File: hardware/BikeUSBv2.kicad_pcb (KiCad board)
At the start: 2 copper layers, 43.6 x 25.5 mm, 53 parts, among them J1 TYPE-C-31-M-16, J2 JST S2B-EH(LF)(SN), SW1 1TS002E-2500-2501-CT, SW2 1TS002E-2500-2501-CT, U1 TPS63020DSJR, U2 ATtiny1616-M, U3 FUSB302B10MPX, U4 HT7550-2, U5 TPS25200

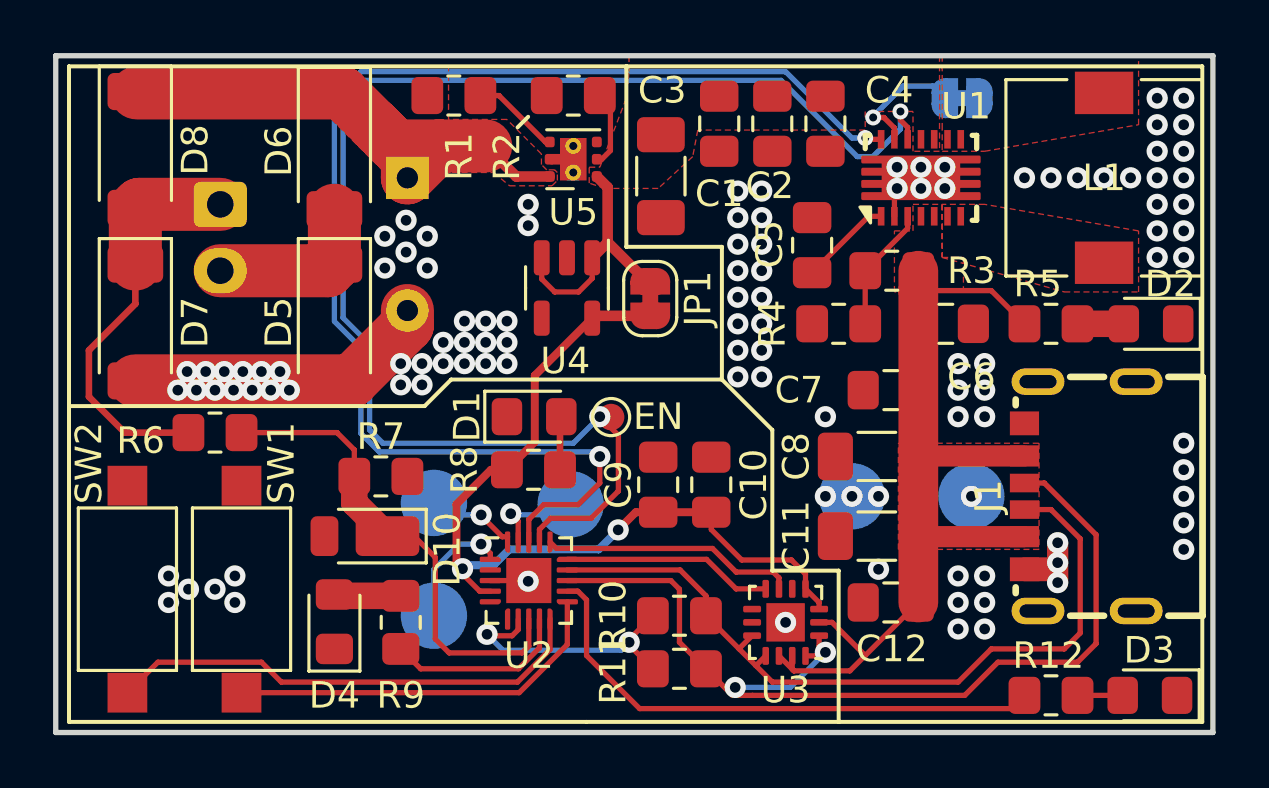
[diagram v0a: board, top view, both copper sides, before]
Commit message: auto cleanup
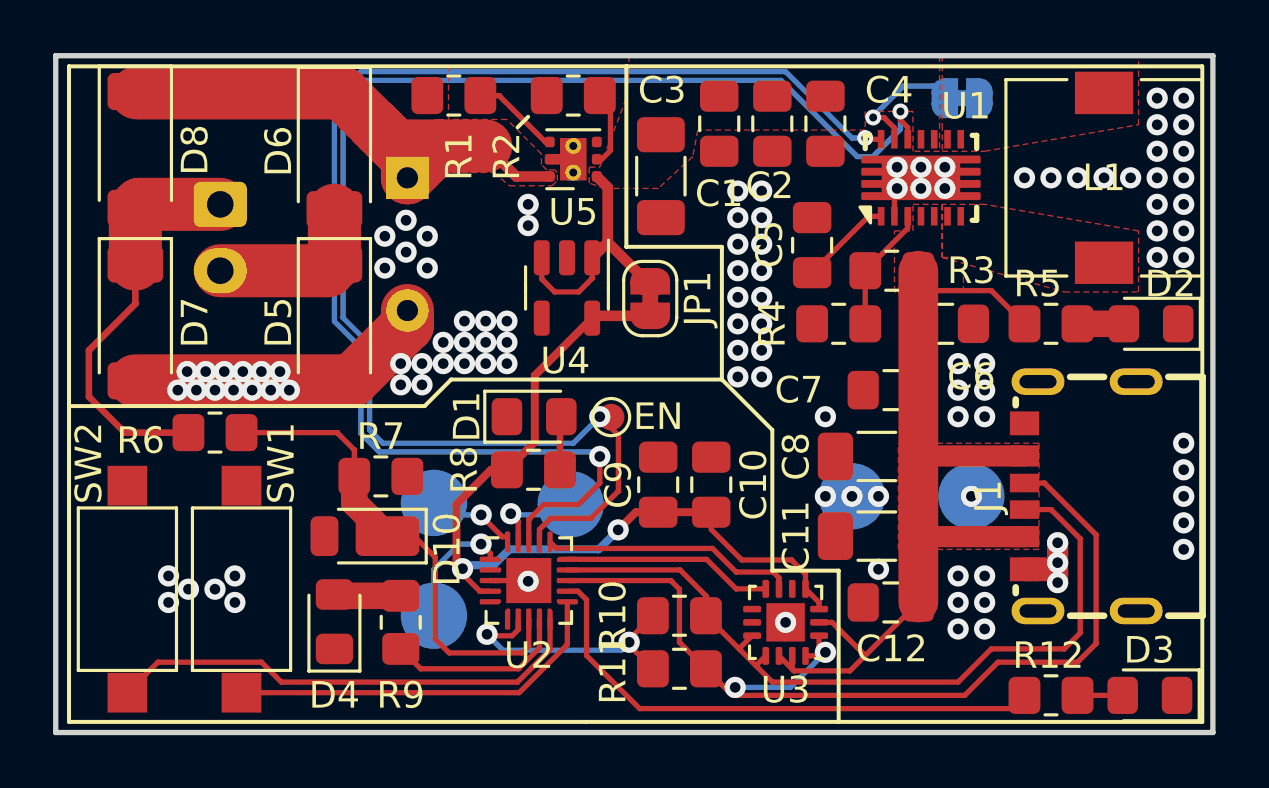
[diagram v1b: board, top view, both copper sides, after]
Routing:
- net Net-(U5-ILIM): track 2.89 -> 2.32 mm
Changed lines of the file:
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@@
   (segment (start 138.7625 103.25) (end 138.7625 103) (width 0.2) (layer "F.Cu") (net 3))
   (segment (start 131.8565 99.6) (end 131.191 100.2655) (width 0.3) (layer "F.Cu") (net 3))
-  (segment (start 130.3 92.2) (end 130.2125 92.2875) (width 0.2) (layer "F.Cu") (net 3))
   (segment (start 138.25 101.928) (end 137.722 101.4) (width 0.2) (layer "F.Cu") (net 3))
   (segment (start 125.975 102.575) (end 125.327 101.927) (width 0.2) (layer "F.Cu") (net 3))
@@
   (segment (start 148.5 105.25) (end 145.5 105.25) (width 0.2) (layer "F.Cu") (net 27))
   (segment (start 149.2 104.55) (end 148.5 105.25) (width 0.2) (layer "F.Cu") (net 27))
-  (segment (start 136.25 106.5) (end 135.5 106.5) (width 0.2) (layer "F.Cu") (net 27))
+  (segment (start 135.5 106.5) (end 144.25 106.5) (width 0.2) (layer "F.Cu") (net 27))
   (segment (start 147.25 98.5) (end 149.2 100.45) (width 0.2) (layer "F.Cu") (net 27))
   (segment (start 149.2 100.45) (end 149.2 104.55) (width 0.2) (layer "F.Cu") (net 27))
   (segment (start 146.5 98.5) (end 147.25 98.5) (width 0.2) (layer "F.Cu") (net 27))
   (segment (start 135.6 106.2) (end 135.6 106.4) (width 0.2) (layer "F.Cu") (net 27))
-  (segment (start 144.25 106.5) (end 136.25 106.5) (width 0.2) (layer "F.Cu") (net 27))
   (segment (start 133.5 102.5) (end 133.175 102.175) (width 0.2) (layer "F.Cu") (net 27))
   (segment (start 138.7625 104.64) (end 139 104.8775) (width 0.2) (layer "F.Cu") (net 27))
@@
   (segment (start 130.795 89.43) (end 130.2125 90.0125) (width 0.4) (layer "F.Cu") (net 36))
   (segment (start 129.7 91.3) (end 128.8 91.3) (width 0.2) (layer "F.Cu") (net 36))
-  (segment (start 132.4 90.9) (end 132.265 90.9) (width 0.4) (layer "F.Cu") (net 36))
   (segment (start 130.3875 86.95) (end 130.795 87.3575) (width 0.4) (layer "F.Cu") (net 36))
   (segment (start 130.2125 90.0125) (end 130.2125 90.7875) (width 0.2) (layer "F.Cu") (net 36))
@@
   (segment (start 130.2125 90.7875) (end 129.7 91.3) (width 0.2) (layer "F.Cu") (net 36))
   (segment (start 128.8 91.3) (end 128.3125 90.8125) (width 0.2) (layer "F.Cu") (net 36))
-  (segment (start 130.9 84.3) (end 130.5 83.9) (width 0.2) (layer "F.Cu") (net 37))
   (segment (start 130.574999 86.3) (end 130.9 85.974999) (width 0.2) (layer "F.Cu") (net 37))
   (segment (start 130.3875 86.3) (end 130.574999 86.3) (width 0.2) (layer "F.Cu") (net 37))
